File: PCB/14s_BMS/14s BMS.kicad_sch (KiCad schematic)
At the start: 0 parts

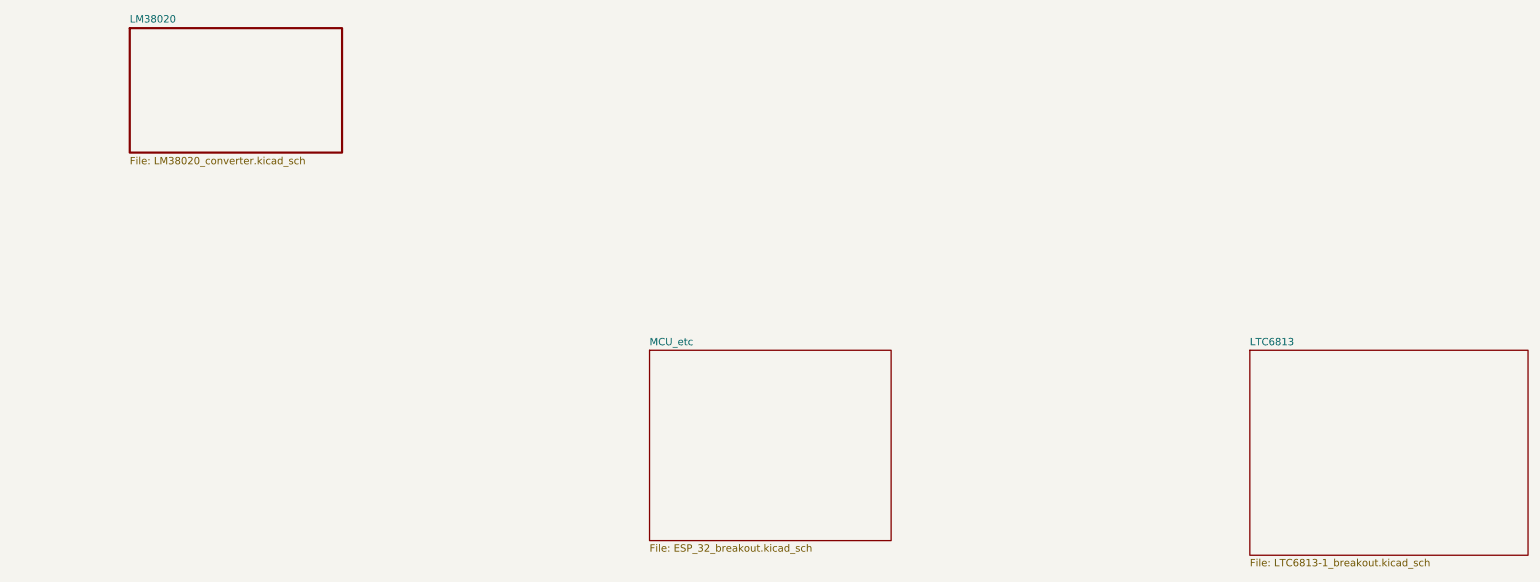
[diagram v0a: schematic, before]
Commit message: rev 1 of power supply design
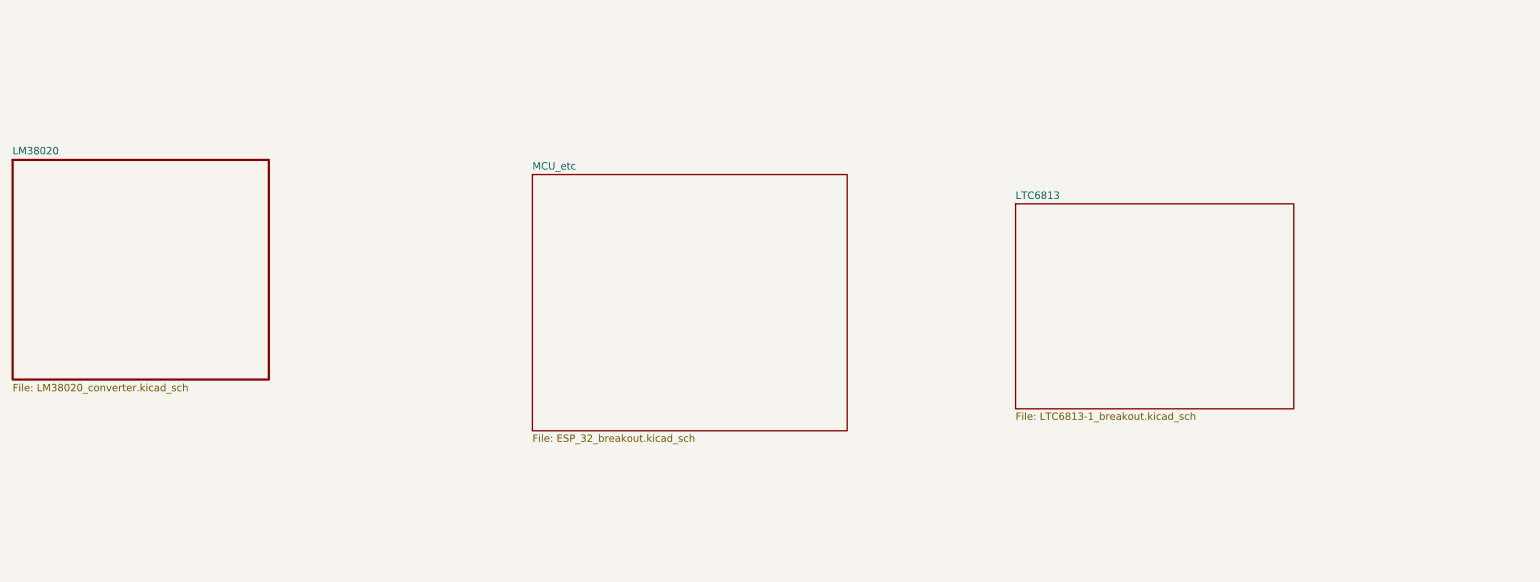
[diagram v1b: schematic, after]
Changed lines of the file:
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@@
 	(generator "eeschema")
 	(generator_version "8.0")
-	(paper "A3")
+	(paper "A4")
 	(sheet
-		(at 43.18 49.53)
-		(size 36.83 21.59)
+		(at 22.86 72.39)
+		(size 44.45 38.1)
 		(fields_autoplaced yes)
 		(stroke
@@
 		)
 		(property "Sheetname" "LM38020"
-			(at 43.18 48.7041 0)
+			(at 22.86 71.5641 0)
 			(effects
 				(font
@@
 		)
 		(property "Sheetfile" "LM38020_converter.kicad_sch"
-			(at 43.18 71.8189 0)
+			(at 22.86 111.1889 0)
 			(effects
 				(font
@@
 	)
 	(sheet
-		(at 133.35 105.41)
-		(size 41.91 33.02)
+		(at 113.03 74.93)
+		(size 54.61 44.45)
 		(fields_autoplaced yes)
 		(stroke
@@
 		)
 		(property "Sheetname" "MCU_etc"
-			(at 133.35 104.6984 0)
+			(at 113.03 74.2184 0)
 			(effects
 				(font
@@
 		)
 		(property "Sheetfile" "ESP_32_breakout.kicad_sch"
-			(at 133.35 139.0146 0)
+			(at 113.03 119.9646 0)
 			(effects
 				(font
@@
 	)
 	(sheet
-		(at 237.49 105.41)
+		(at 196.85 80.01)
 		(size 48.26 35.56)
 		(fields_autoplaced yes)
@@
 		)
 		(property "Sheetname" "LTC6813"
-			(at 237.49 104.6984 0)
+			(at 196.85 79.2984 0)
 			(effects
 				(font
@@
 		)
 		(property "Sheetfile" "LTC6813-1_breakout.kicad_sch"
-			(at 237.49 141.5546 0)
+			(at 196.85 116.1546 0)
 			(effects
 				(font
